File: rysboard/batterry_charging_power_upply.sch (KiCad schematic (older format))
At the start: 7 parts, among them J7 Conn_01x02, Q6 Si7938DP-T1-GE3, U8 LM74700

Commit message: Bom finished pcb cleanup started
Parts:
- removed D16: PTVS30VS1UR,115, Diode_SMD:D_SOD-123, symbol Device:D_TVS
- removed U8: LM74700, Package_TO_SOT_SMD:SOT-23-6, symbol Power_Management:LM74700
- added IC2: LM74801QDRRRQ1, LM74801QDRRRQ1, symbol SamacSys_Parts:LM74801QDRRRQ1
- added R32: 100R, Resistor_SMD:R_0603_1608Metric, symbol Device:R
- F2: footprint Fuse:Fuse_2512_6332Metric -> Fuse:Fuse_1206_3216Metric
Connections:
- net labels added: DC_IN_Voltage
- net labels removed: VCAP
- wire segments 19 -> 31
- no-connect marks 0 -> 2
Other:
- moved on the sheet: C31, F2
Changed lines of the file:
@@
 L Device:Fuse F2
 U 1 1 5FF0CA02
-P 2525 1475
-F 0 "F2" V 2328 1475 50  0000 C CNN
-F 1 "Fuse" V 2419 1475 50  0000 C CNN
-F 2 "Fuse:Fuse_2512_6332Metric" V 2455 1475 50  0001 C CNN
-F 3 "~" H 2525 1475 50  0001 C CNN
-	1    2525 1475
+P 2575 1175
+F 0 "F2" V 2378 1175 50  0000 C CNN
+F 1 "Fuse" V 2469 1175 50  0000 C CNN
+F 2 "Fuse:Fuse_1206_3216Metric" V 2505 1175 50  0001 C CNN
+F 3 "~" H 2575 1175 50  0001 C CNN
+	1    2575 1175
 	0    1    1    0
 $EndComp
@@
 P 3250 1625
 F 0 "C34" H 3175 1525 50  0000 L CNN
-F 1 "10uF" H 3150 1375 50  0000 L CNN
+F 1 "10uF" H 3550 1650 50  0000 L CNN
 F 2 "Capacitor_SMD:C_1206_3216Metric" H 3288 1475 50  0001 C CNN
 F 3 "~" H 3250 1625 50  0001 C CNN
@@
 Text Notes 3050 1000 0    50   ~ 0
 REMOVE ADDITIONA L mosfet USE INTERNAL SHUDTOWN PIN
-$Comp
-L Power_Management:LM74700 U8
-U 1 1 6056EF72
-P 4750 2275
-F 0 "U8" H 5180 2321 50  0000 L CNN
-F 1 "LM74700" H 5180 2230 50  0000 L CNN
-F 2 "Package_TO_SOT_SMD:SOT-23-6" H 4375 1925 50  0001 C CNN
-F 3 "http://www.ti.com/lit/gpn/LM74700-Q1" H 4375 1925 50  0001 C CNN
-	1    4750 2275
-	1    0    0    -1
-$EndComp
 Wire Wire Line
 	4750 1775 4750 1875
-Wire Wire Line
-	4550 1475 4450 1475
-Wire Wire Line
-	4450 1475 4450 1875
-Wire Wire Line
-	4950 1475 5050 1475
-Wire Wire Line
-	5050 1475 5050 1875
-Connection ~ 5050 1475
-Connection ~ 4450 1475
 $Comp
 L power:GND #PWR040
 U 1 1 60572C01
-P 4750 2900
-F 0 "#PWR040" H 4750 2650 50  0001 C CNN
-F 1 "GND" H 4755 2727 50  0000 C CNN
-F 2 "" H 4750 2900 50  0001 C CNN
-F 3 "" H 4750 2900 50  0001 C CNN
-	1    4750 2900
+P 5150 3325
+F 0 "#PWR040" H 5150 3075 50  0001 C CNN
+F 1 "GND" H 5155 3152 50  0000 C CNN
+F 2 "" H 5150 3325 50  0001 C CNN
+F 3 "" H 5150 3325 50  0001 C CNN
+	1    5150 3325
 	1    0    0    -1
 $EndComp
-Wire Wire Line
-	4750 2900 4750 2675
 $Comp
 L Device:C C31
 U 1 1 60573158
-P 6625 2300
-F 0 "C31" H 6475 2400 50  0000 L CNN
-F 1 "0.1uF" H 6300 2300 50  0000 L CNN
-F 2 "Capacitor_SMD:C_0603_1608Metric" H 6663 2150 50  0001 C CNN
-F 3 "~" H 6625 2300 50  0001 C CNN
-	1    6625 2300
-	1    0    0    -1
+P 5125 1750
+F 0 "C31" H 4975 1850 50  0000 L CNN
+F 1 "0.1uF" V 5275 1650 50  0000 L CNN
+F 2 "Capacitor_SMD:C_0603_1608Metric" H 5163 1600 50  0001 C CNN
+F 3 "~" H 5125 1750 50  0001 C CNN
+	1    5125 1750
+	0    1    1    0
 $EndComp
-Wire Wire Line
-	3650 1475 4450 1475
-Wire Wire Line
-	3650 2475 4250 2475
 $Comp
 L power:GND #PWR042
 U 1 1 60574E8B
-P 6625 2450
-F 0 "#PWR042" H 6625 2200 50  0001 C CNN
-F 1 "GND" H 6630 2277 50  0000 C CNN
-F 2 "" H 6625 2450 50  0001 C CNN
-F 3 "" H 6625 2450 50  0001 C CNN
-	1    6625 2450
+P 5925 2500
+F 0 "#PWR042" H 5925 2250 50  0001 C CNN
+F 1 "GND" H 5930 2327 50  0000 C CNN
+F 2 "" H 5925 2500 50  0001 C CNN
+F 3 "" H 5925 2500 50  0001 C CNN
+	1    5925 2500
 	1    0    0    -1
 $EndComp
-Text Label 4050 2375 0    50   ~ 0
-VCAP
-Wire Wire Line
-	4050 2375 4250 2375
-Text Label 6425 2150 0    50   ~ 0
-VCAP
-Wire Wire Line
-	6425 2150 6625 2150
-Wire Wire Line
-	2675 1475 2725 1475
-Wire Wire Line
-	3250 1475 3650 1475
-Connection ~ 3250 1475
-Connection ~ 3650 1475
-$Comp
-L Device:D_TVS D16
-U 1 1 6057AB93
-P 2725 1625
-F 0 "D16" V 2679 1705 50  0000 L CNN
-F 1 "PTVS30VS1UR,115 " V 2770 1705 50  0000 L CNN
-F 2 "Diode_SMD:D_SOD-123" H 2725 1625 50  0001 C CNN
-F 3 "~" H 2725 1625 50  0001 C CNN
-	1    2725 1625
-	0    1    1    0
-$EndComp
-Connection ~ 2725 1475
-Wire Wire Line
-	2725 1475 3250 1475
 Wire Wire Line
 	3250 1775 2725 1775
@@
 TODO -16 V Vmax\n
 Wire Wire Line
-	3650 1475 3650 2475
+	2425 1175 2375 1175
 Wire Wire Line
-	5050 1475 6250 1475
+	2375 1175 2375 1475
+Wire Wire Line
+	2725 1175 3250 1175
+Wire Wire Line
+	3250 1175 3250 1475
+Connection ~ 3250 1475
+$Comp
+L SamacSys_Parts:LM74801QDRRRQ1 IC2
+U 1 1 60A0C1A8
+P 5250 2500
+F 0 "IC2" H 5200 2500 50  0000 C CNN
+F 1 "LM74801QDRRRQ1" H 5225 2275 50  0000 C CNN
+F 2 "LM74801QDRRRQ1" H 6400 2600 50  0001 L CNN
+F 3 "https://www.ti.com/lit/gpn/LM7480-Q1" H 6400 2500 50  0001 L CNN
+F 4 "3-V TO 65-V, AUTOMOTIVE IDEAL DI" H 6400 2400 50  0001 L CNN "Description"
+F 5 "0.8" H 6400 2300 50  0001 L CNN "Height"
+F 6 "595-LM74801QDRRRQ1" H 6400 2200 50  0001 L CNN "Mouser Part Number"
+F 7 "https://www.mouser.co.uk/ProductDetail/Texas-Instruments/LM74801QDRRRQ1?qs=zW32dvEIR3uHxOfYWHY8FQ%3D%3D" H 6400 2100 50  0001 L CNN "Mouser Price/Stock"
+F 8 "Texas Instruments" H 6400 2000 50  0001 L CNN "Manufacturer_Name"
+F 9 "LM74801QDRRRQ1" H 6400 1900 50  0001 L CNN "Manufacturer_Part_Number"
+	1    5250 2500
+	1    0    0    -1
+$EndComp
+Wire Wire Line
+	4375 2350 4375 1475
+Connection ~ 4375 1475
+Wire Wire Line
+	4375 1475 4550 1475
+Wire Wire Line
+	4950 1475 5400 1475
+Wire Wire Line
+	4975 1750 4950 1750
+Wire Wire Line
+	4950 1750 4950 1875
+Wire Wire Line
+	5275 1750 5300 1750
+Wire Wire Line
+	5300 1750 5300 1875
+Wire Wire Line
+	5300 1750 5400 1750
+Wire Wire Line
+	5400 1750 5400 1875
+Connection ~ 5300 1750
+Wire Wire Line
+	5400 1750 5400 1475
+Connection ~ 5400 1750
+Connection ~ 5400 1475
+Wire Wire Line
+	5400 1475 6250 1475
+NoConn ~ 5600 1875
+Wire Wire Line
+	4375 2350 4375 2450
+Connection ~ 4375 2350
+Wire Wire Line
+	3250 1475 4375 1475
+NoConn ~ 4400 2800
+$Comp
+L Device:R R32
+U 1 1 60A1425A
+P 4050 2675
+F 0 "R32" H 4120 2721 50  0000 L CNN
+F 1 "100R" H 4120 2630 50  0000 L CNN
+F 2 "Resistor_SMD:R_0603_1608Metric" V 3980 2675 50  0001 C CNN
+F 3 "~" H 4050 2675 50  0001 C CNN
+	1    4050 2675
+	1    0    0    -1
+$EndComp
+$Comp
+L power:GND #PWR025
+U 1 1 60A14B90
+P 4250 3125
+F 0 "#PWR025" H 4250 2875 50  0001 C CNN
+F 1 "GND" H 4255 2952 50  0000 C CNN
+F 2 "" H 4250 3125 50  0001 C CNN
+F 3 "" H 4250 3125 50  0001 C CNN
+	1    4250 3125
+	1    0    0    -1
+$EndComp
+Wire Wire Line
+	4050 2525 4225 2525
+Wire Wire Line
+	4225 2525 4225 2550
+Wire Wire Line
+	4225 2550 4375 2550
+Wire Wire Line
+	3650 2825 4050 2825
+Wire Wire Line
+	4250 3125 4250 3050
+Wire Wire Line
+	4250 3050 4400 3050
+Text GLabel 3650 2825 0    50   Input ~ 0
+DC_IN_Voltage
+Wire Wire Line
+	5400 1750 6275 1750
+Wire Wire Line
+	6275 1750 6275 2875
+Wire Wire Line
+	6275 2875 5925 2875
 $EndSCHEMATC

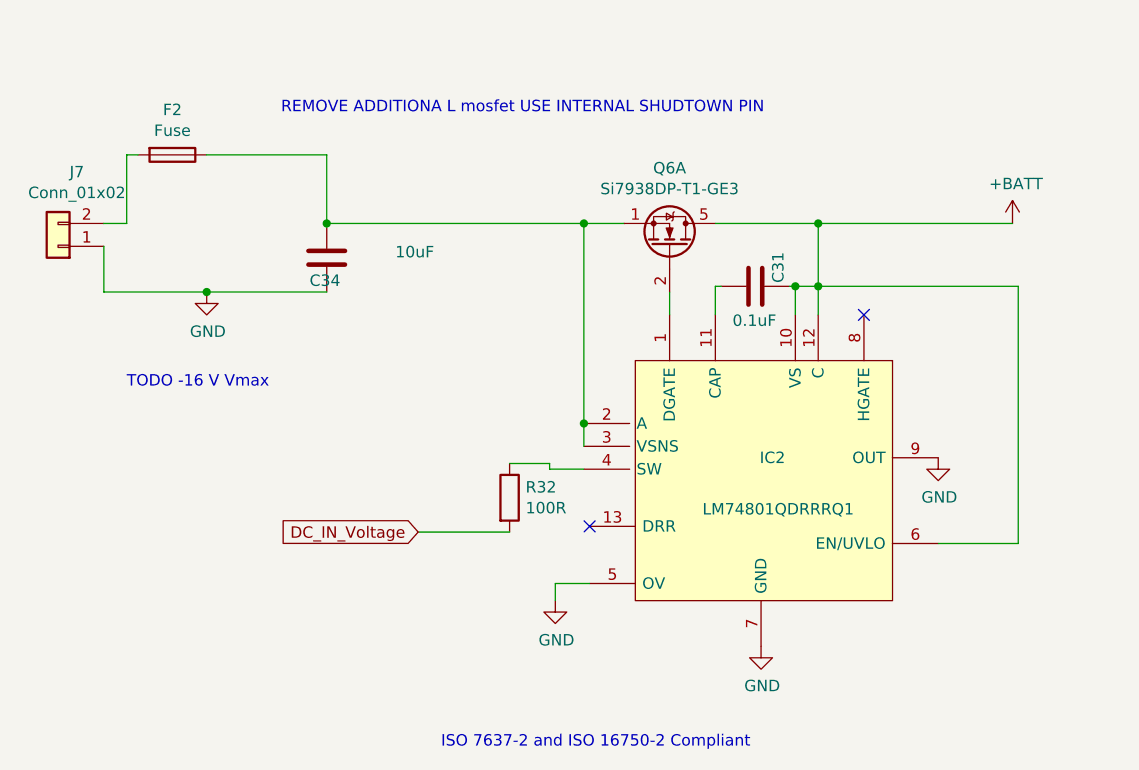
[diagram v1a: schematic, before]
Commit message: bom + excel ready
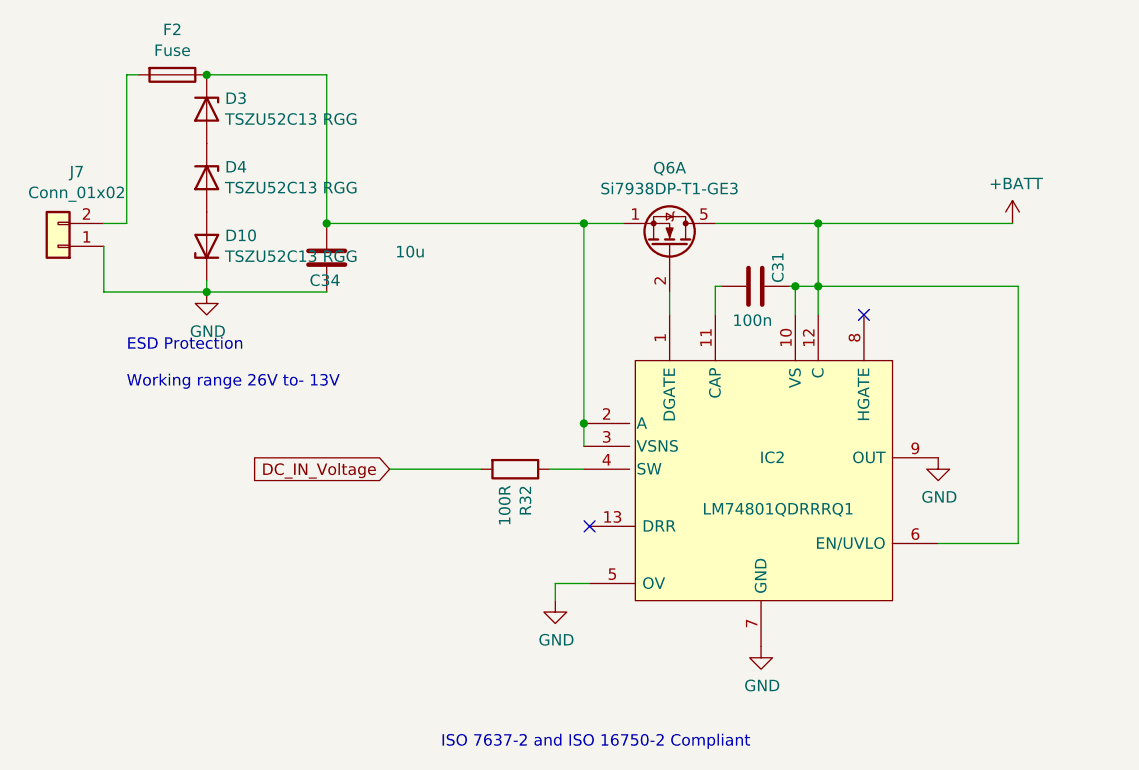
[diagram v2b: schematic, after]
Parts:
- added D10, D3, D4: TSZU52C13 RGG, Diode_SMD:D_0603_1608Metric, symbol Device:D_Zener
- C31: value 0.1uF -> 100n
- C34: value 10uF -> 10u
- IC2: footprint LM74801QDRRRQ1 -> SamacSys_Parts:LM74801QDRRRQ1
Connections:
- net GND: now also D10.1 (K)
- net at C34.1, F2.1, IC2.2 (A)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: now also D3.1 (K)
- new net: D3.2 (A), D4.1 (K)
- new net: D10.2 (A), D4.2 (A)
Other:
- note added: "ESD Protection\n\nWorking range 26V to- 13V\n"
- note removed: "REMOVE ADDITIONA L mosfet USE INTERNAL SHUDTOWN PIN"
- note removed: "TODO -16 V Vmax\n"
- moved on the sheet: F2, R32
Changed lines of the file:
@@
 L Device:Fuse F2
 U 1 1 5FF0CA02
-P 2575 1175
-F 0 "F2" V 2378 1175 50  0000 C CNN
-F 1 "Fuse" V 2469 1175 50  0000 C CNN
-F 2 "Fuse:Fuse_1206_3216Metric" V 2505 1175 50  0001 C CNN
-F 3 "~" H 2575 1175 50  0001 C CNN
-	1    2575 1175
+P 2575 825
+F 0 "F2" V 2378 825 50  0000 C CNN
+F 1 "Fuse" V 2469 825 50  0000 C CNN
+F 2 "Fuse:Fuse_1206_3216Metric" V 2505 825 50  0001 C CNN
+F 3 "~" H 2575 825 50  0001 C CNN
+	1    2575 825
 	0    1    1    0
 $EndComp
@@
 P 3250 1625
 F 0 "C34" H 3175 1525 50  0000 L CNN
-F 1 "10uF" H 3550 1650 50  0000 L CNN
+F 1 "10u" H 3550 1650 50  0000 L CNN
 F 2 "Capacitor_SMD:C_1206_3216Metric" H 3288 1475 50  0001 C CNN
 F 3 "~" H 3250 1625 50  0001 C CNN
@@
 Wire Wire Line
 	2375 1475 2275 1475
-Text Notes 3050 1000 0    50   ~ 0
-REMOVE ADDITIONA L mosfet USE INTERNAL SHUDTOWN PIN
 Wire Wire Line
 	4750 1775 4750 1875
@@
 P 5125 1750
 F 0 "C31" H 4975 1850 50  0000 L CNN
-F 1 "0.1uF" V 5275 1650 50  0000 L CNN
+F 1 "100n" V 5275 1650 50  0000 L CNN
 F 2 "Capacitor_SMD:C_0603_1608Metric" H 5163 1600 50  0001 C CNN
 F 3 "~" H 5125 1750 50  0001 C CNN
@@
 	1    0    0    -1
 $EndComp
-Wire Wire Line
-	3250 1775 2725 1775
 Wire Wire Line
 	2275 1775 2275 1575
@@
 $EndComp
 Text Notes 2375 2200 0    50   ~ 0
-TODO -16 V Vmax\n
-Wire Wire Line
-	2425 1175 2375 1175
-Wire Wire Line
-	2375 1175 2375 1475
-Wire Wire Line
-	2725 1175 3250 1175
-Wire Wire Line
-	3250 1175 3250 1475
+ESD Protection\n\nWorking range 26V to- 13V\n
 Connection ~ 3250 1475
 $Comp
@@
 F 0 "IC2" H 5200 2500 50  0000 C CNN
 F 1 "LM74801QDRRRQ1" H 5225 2275 50  0000 C CNN
-F 2 "LM74801QDRRRQ1" H 6400 2600 50  0001 L CNN
+F 2 "SamacSys_Parts:LM74801QDRRRQ1" H 6400 2600 50  0001 L CNN
 F 3 "https://www.ti.com/lit/gpn/LM7480-Q1" H 6400 2500 50  0001 L CNN
 F 4 "3-V TO 65-V, AUTOMOTIVE IDEAL DI" H 6400 2400 50  0001 L CNN "Description"
@@
 L Device:R R32
 U 1 1 60A1425A
-P 4050 2675
-F 0 "R32" H 4120 2721 50  0000 L CNN
-F 1 "100R" H 4120 2630 50  0000 L CNN
-F 2 "Resistor_SMD:R_0603_1608Metric" V 3980 2675 50  0001 C CNN
-F 3 "~" H 4050 2675 50  0001 C CNN
-	1    4050 2675
-	1    0    0    -1
+P 4075 2550
+F 0 "R32" H 4145 2596 50  0000 L CNN
+F 1 "100R" H 4145 2505 50  0000 L CNN
+F 2 "Resistor_SMD:R_0603_1608Metric" V 4005 2550 50  0001 C CNN
+F 3 "~" H 4075 2550 50  0001 C CNN
+	1    4075 2550
+	0    1    1    0
 $EndComp
 $Comp
@@
 $EndComp
 Wire Wire Line
-	4050 2525 4225 2525
-Wire Wire Line
-	4225 2525 4225 2550
-Wire Wire Line
 	4225 2550 4375 2550
 Wire Wire Line
-	3650 2825 4050 2825
+	3525 2550 3925 2550
 Wire Wire Line
 	4250 3125 4250 3050
 Wire Wire Line
 	4250 3050 4400 3050
-Text GLabel 3650 2825 0    50   Input ~ 0
+Text GLabel 3525 2550 0    50   Input ~ 0
 DC_IN_Voltage
 Wire Wire Line
@@
 Wire Wire Line
 	6275 2875 5925 2875
+$Comp
+L Device:D_Zener D3
+U 1 1 60911B5B
+P 2725 975
+F 0 "D3" V 2679 1055 50  0000 L CNN
+F 1 "TSZU52C13 RGG " V 2770 1055 50  0000 L CNN
+F 2 "Diode_SMD:D_0603_1608Metric" H 2725 975 50  0001 C CNN
+F 3 "~" H 2725 975 50  0001 C CNN
+	1    2725 975
+	0    1    1    0
+$EndComp
+$Comp
+L Device:D_Zener D4
+U 1 1 60929F45
+P 2725 1275
+F 0 "D4" V 2679 1355 50  0000 L CNN
+F 1 "TSZU52C13 RGG " V 2770 1355 50  0000 L CNN
+F 2 "Diode_SMD:D_0603_1608Metric" H 2725 1275 50  0001 C CNN
+F 3 "~" H 2725 1275 50  0001 C CNN
+	1    2725 1275
+	0    1    1    0
+$EndComp
+$Comp
+L Device:D_Zener D10
+U 1 1 6092B35B
+P 2725 1575
+F 0 "D10" V 2771 1495 50  0000 R CNN
+F 1 "TSZU52C13 RGG " V 2680 1495 50  0000 R CNN
+F 2 "Diode_SMD:D_0603_1608Metric" H 2725 1575 50  0001 C CNN
+F 3 "~" H 2725 1575 50  0001 C CNN
+	1    2725 1575
+	0    -1   -1   0
+$EndComp
+Wire Wire Line
+	2725 1725 2725 1775
+Wire Wire Line
+	2725 1775 3250 1775
+Wire Wire Line
+	3250 825  2725 825
+Wire Wire Line
+	3250 825  3250 1475
+Connection ~ 2725 825
+Wire Wire Line
+	2425 825  2375 825
+Wire Wire Line
+	2375 825  2375 1475
 $EndSCHEMATC

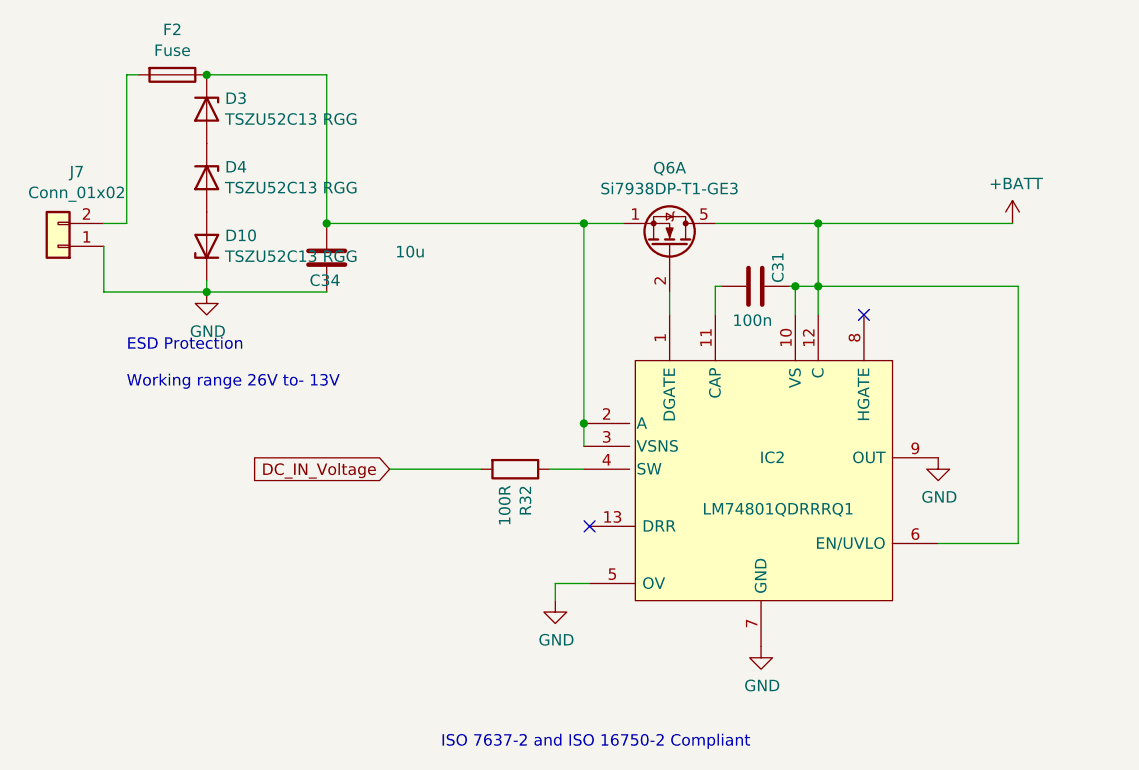
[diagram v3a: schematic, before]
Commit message: New Layout done TODo Error Check
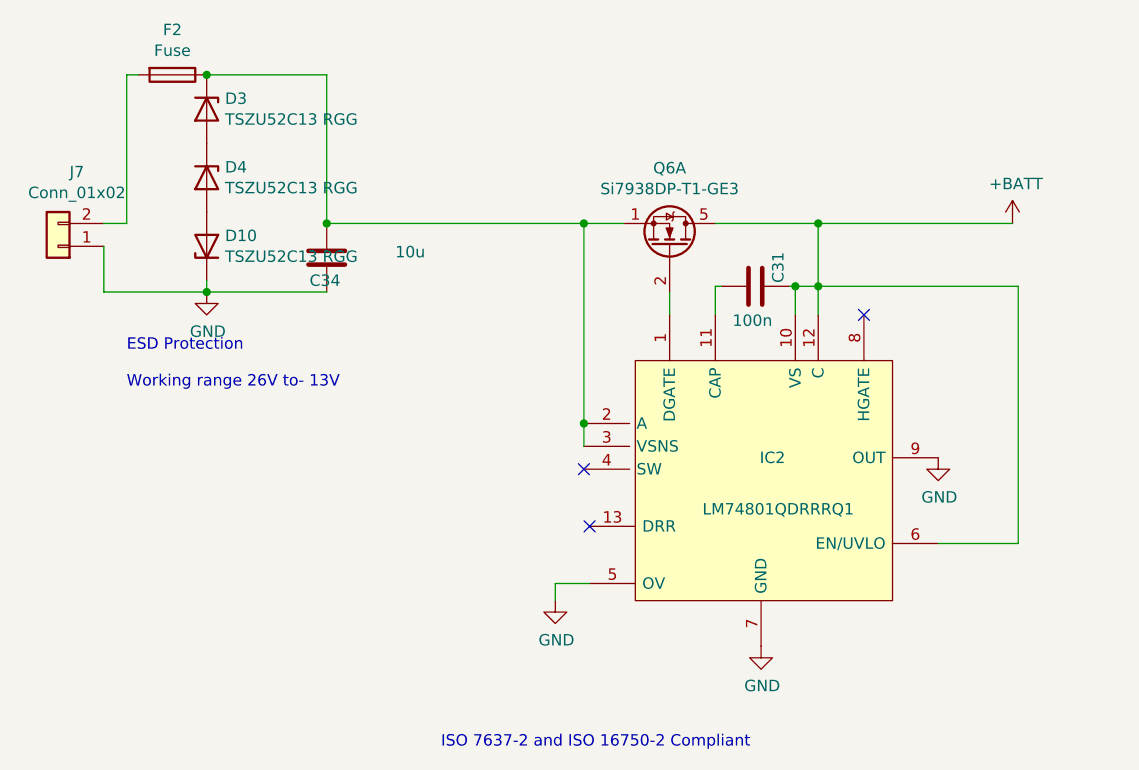
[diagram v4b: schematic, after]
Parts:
- removed R32: 100R, Resistor_SMD:R_0603_1608Metric, symbol Device:R
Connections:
- no-connect marks 2 -> 3
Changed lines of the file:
@@
 Wire Wire Line
 	2375 825  2375 1475
-Wire Wire Line
-	4225 2550 4375 2550
-Wire Wire Line
-	3525 2550 3925 2550
-Text GLabel 3525 2550 0    50   Input ~ 0
-DC_IN_Voltage
-$Comp
-L Device:R R32
-U 1 1 60A1425A
-P 4075 2550
-F 0 "R32" H 4145 2596 50  0000 L CNN
-F 1 "100R" H 4145 2505 50  0000 L CNN
-F 2 "Resistor_SMD:R_0603_1608Metric" V 4005 2550 50  0001 C CNN
-F 3 "~" H 4075 2550 50  0001 C CNN
-	1    4075 2550
-	0    1    1    0
-$EndComp
+NoConn ~ 4375 2550
 $EndSCHEMATC
